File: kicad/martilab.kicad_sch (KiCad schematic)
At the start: 9 parts, among them J1 Conn_01x20, J2 Conn_01x20, J3 Conn_01x02, Q2 BS250, SW1 SW_Push, U1 Pico, U2 DFR0299, U3 RTC DS1307

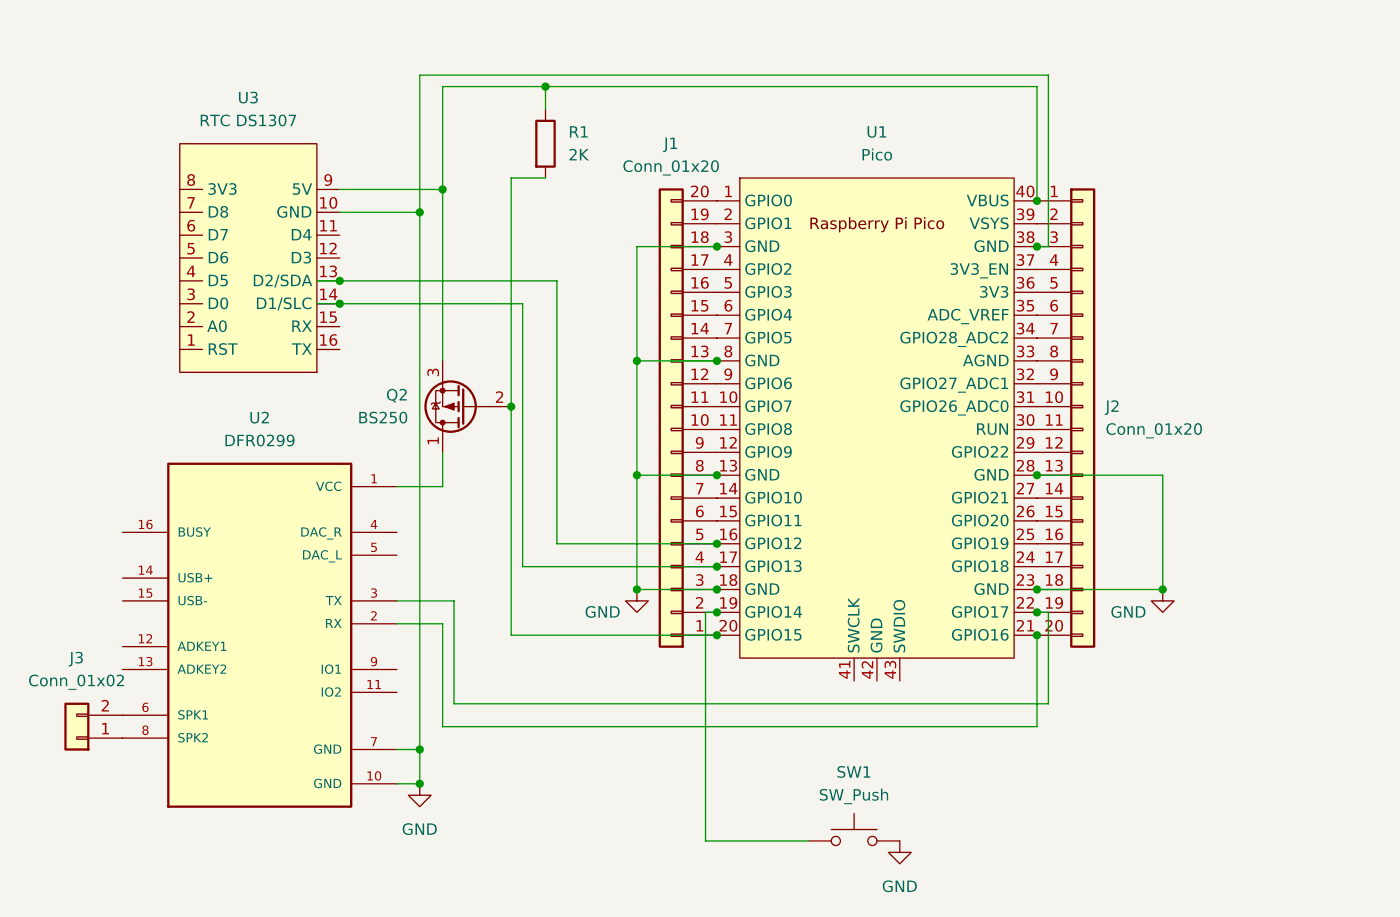
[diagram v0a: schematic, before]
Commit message: add schema
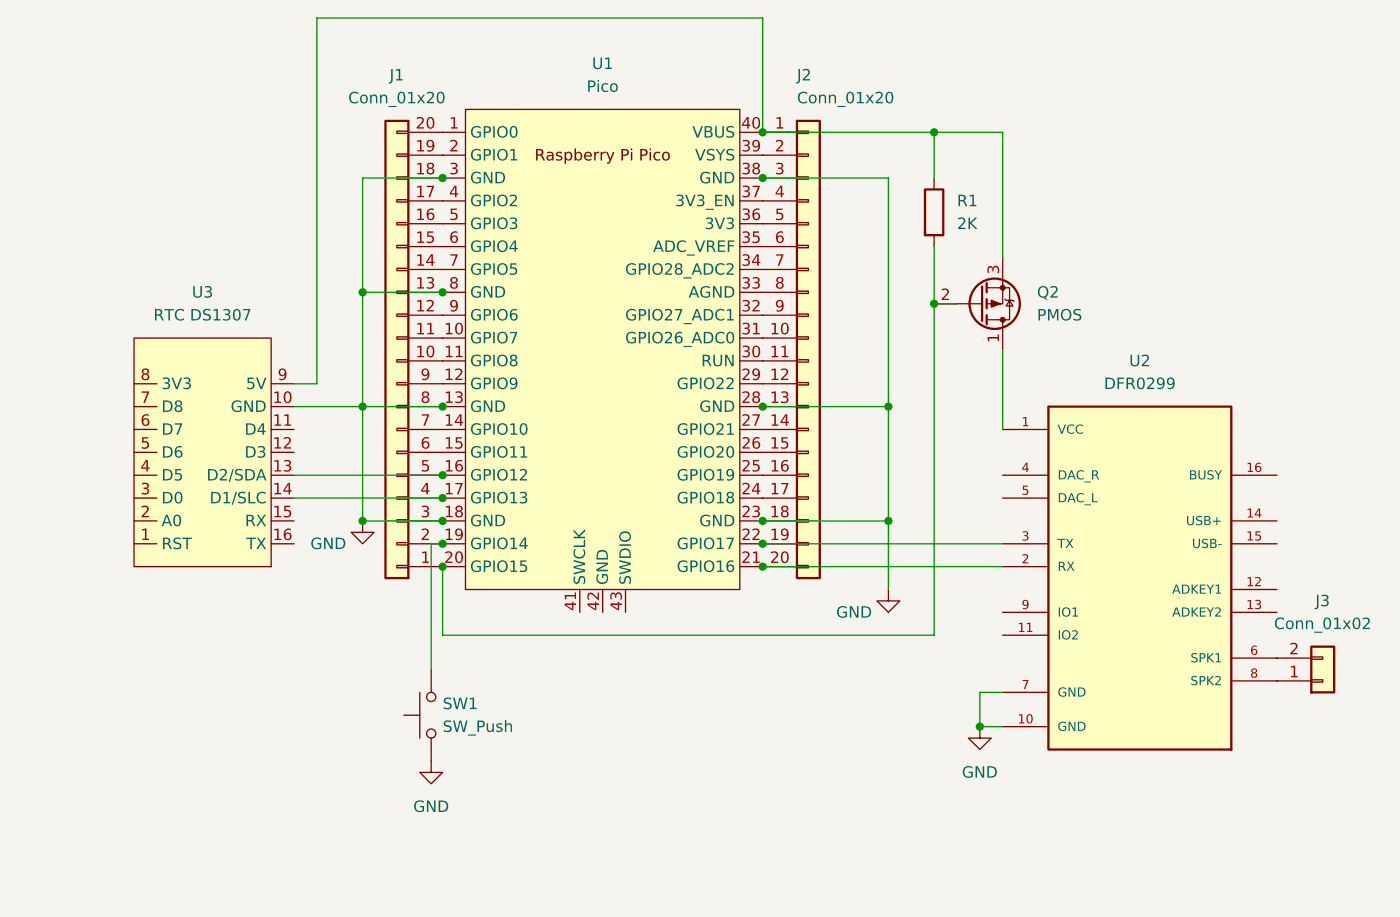
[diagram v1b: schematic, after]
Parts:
- Q2: value BS250 -> PMOS
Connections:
- net GND: now also SW1.1; no longer SW1.2
- net at J1.2 (Pin_2), U1.19 (GPIO14): now also SW1.2; no longer SW1.1
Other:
- moved on the sheet: J1, J2, J3, Q2, R1, SW1, U1, U2, U3
